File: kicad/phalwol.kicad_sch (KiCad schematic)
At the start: 85 parts, among them J1 AudioJack4, SW1 SW_Push, SW10 SW_Push, SW11 SW_Push, SW12 SW_Push, SW13 SW_Push, SW14 SW_Push, SW15 SW_Push, SW16 SW_Push, SW17 SW_Push, SW18 SW_Push, SW19 SW_Push, SW2 SW_Push, SW20 SW_Push, SW21 SW_Push, SW22 SW_Push, SW23 SW_Push, SW24 SW_Push, SW25 SW_Push, SW26 SW_Push, SW27 SW_Push, SW28 SW_Push, SW29 SW_Push, SW3 SW_Push, SW30 SW_Push, SW31 SW_Push, SW32 SW_Push, SW33 SW_Push, SW34 SW_Push, SW35 SW_Push, SW36 SW_Push, SW37 SW_Push, SW38 SW_Push, SW39 SW_Push, SW4 SW_Push, SW40 SW_Push, SW41 SW_Push, SW5 SW_Push, SW6 SW_Push, SW7 SW_Push, SW8 SW_Push, SW9 SW_Push, U1 ProMicro

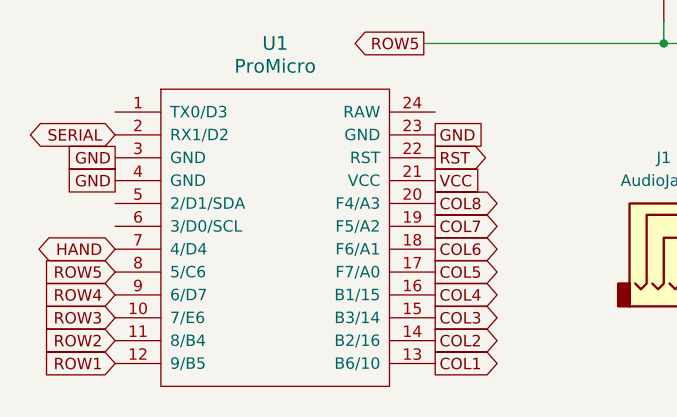
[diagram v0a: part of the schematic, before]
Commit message: hotfix wiring
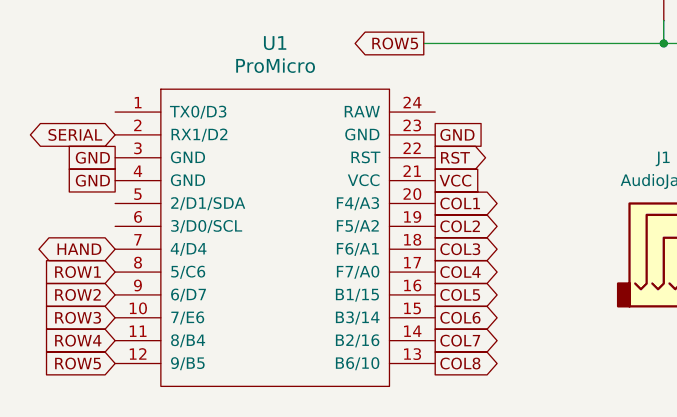
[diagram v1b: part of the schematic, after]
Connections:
- net COL1: now also U1.20 (F4/A3); no longer U1.13 (B6/10)
- net COL2: now also U1.19 (F5/A2); no longer U1.14 (B2/16)
- net COL3: now also U1.18 (F6/A1); no longer U1.15 (B3/14)
- net COL4: now also U1.17 (F7/A0); no longer U1.16 (B1/15)
- net COL5: now also U1.16 (B1/15); no longer U1.17 (F7/A0)
- net COL6: now also U1.15 (B3/14); no longer U1.18 (F6/A1)
- net COL7: now also U1.14 (B2/16); no longer U1.19 (F5/A2)
- net COL8: now also U1.13 (B6/10); no longer U1.20 (F4/A3)
- net ROW1: now also U1.8 (5/C6); no longer U1.12 (9/B5)
- net ROW2: now also U1.9 (6/D7); no longer U1.11 (8/B4)
- net ROW4: now also U1.11 (8/B4); no longer U1.9 (6/D7)
- net ROW5: now also U1.12 (9/B5); no longer U1.8 (5/C6)
